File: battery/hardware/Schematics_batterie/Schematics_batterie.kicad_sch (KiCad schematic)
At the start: 45 parts, among them IC1 BQ25185DLHR, J1 USB_C_Receptacle_USB2.0_16P, J2 Conn_01x02, J3 Conn_01x02, J4 Conn_ST_STDC14, J5 Conn_01x02, U1 BU33SD5WG-TR, U2 STM32G431KBTx, U3 USBLC6-2SC6

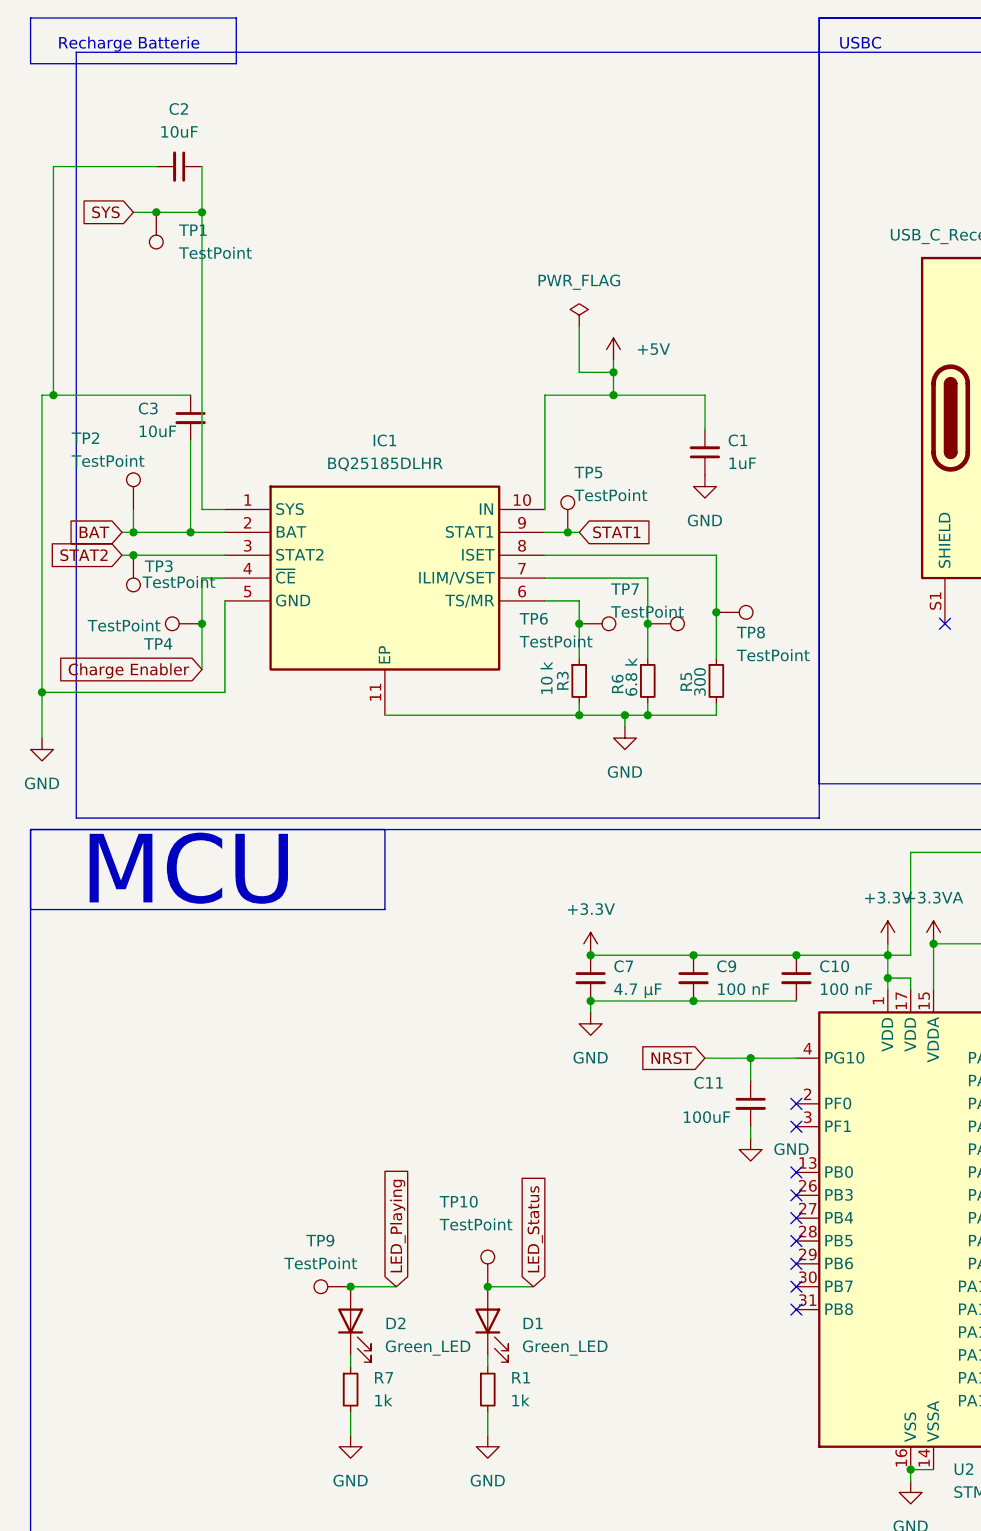
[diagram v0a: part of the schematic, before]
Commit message: derniers branchements et isolation des textes
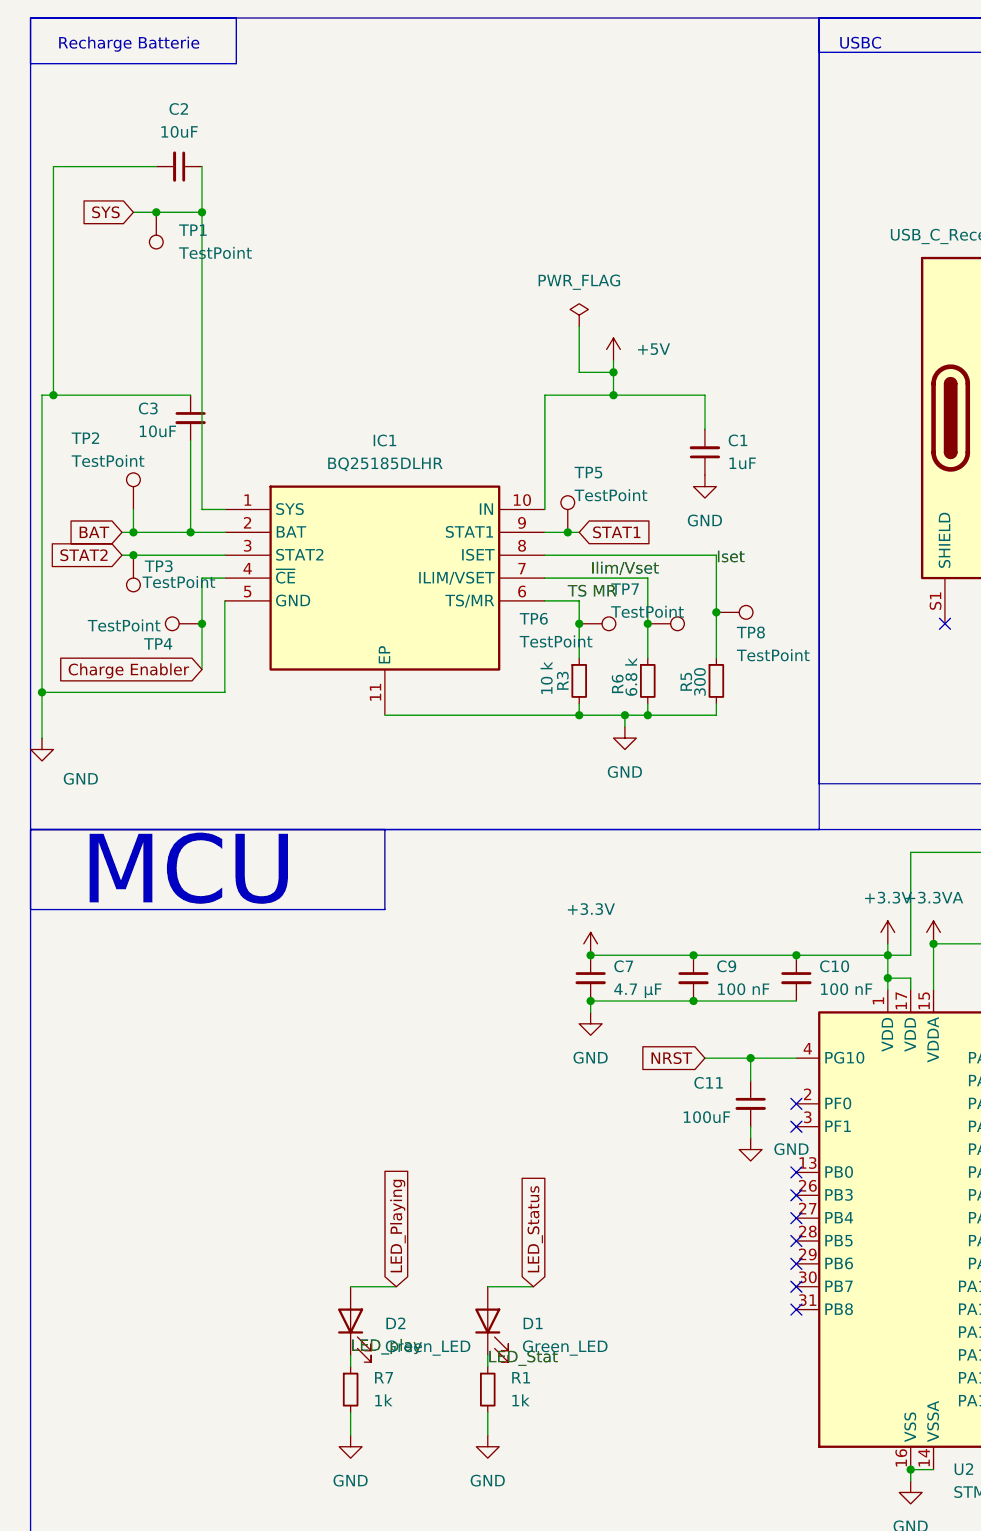
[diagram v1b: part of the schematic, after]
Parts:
- removed TP10, TP9: TestPoint, TestPoint:TestPoint_Pad_D2.0mm, symbol Connector:TestPoint
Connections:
- net TS MR: now reaches IC1.6 (TS/MR), R3.1, TP6.1
- net LED_play: now reaches D2.1 (K), R7.1
- net Ilim/Vset: now reaches IC1.7 (ILIM/VSET), R6.1, TP7.1
- net Iset: now reaches IC1.8 (ISET), R5.1, TP8.1
- net LED_Stat: now reaches D1.1 (K), R1.1
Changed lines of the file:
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@@
 	)
 	(junction
-		(at 55.88 163.83)
-		(diameter 0)
-		(color 0 0 0 0)
-	)
-	(junction
 		(at 100.33 138.43)
 		(diameter 0)
@@
 	)
 	(junction
-		(at 71.12 163.83)
-		(diameter 0)
-		(color 0 0 0 0)
-	)
-	(junction
 		(at 250.19 154.94)
 		(diameter 0)
@@
 	)
 	(rectangle
-		(start 25.4 26.67)
-		(end 107.95 111.76)
+		(start 20.32 22.86)
+		(end 107.95 113.03)
 		(stroke
 			(width 0)
@@
 		)
 	)
+	(label "Ilim{slash}Vset"
+		(at 82.55 85.09 0)
+		(effects
+			(font
+				(size 1.27 1.27)
+			)
+			(justify left bottom)
+		)
+	)
+	(label "TS MR"
+		(at 80.01 87.63 0)
+		(effects
+			(font
+				(size 1.27 1.27)
+			)
+			(justify left bottom)
+		)
+	)
+	(label "LED_Stat"
+		(at 71.12 172.72 0)
+		(effects
+			(font
+				(size 1.27 1.27)
+			)
+			(justify left bottom)
+		)
+	)
 	(label "VIN"
 		(at 187.96 133.35 0)
@@
 		)
 	)
+	(label "Iset"
+		(at 96.52 83.82 0)
+		(effects
+			(font
+				(size 1.27 1.27)
+			)
+			(justify left bottom)
+		)
+	)
+	(label "LED_play"
+		(at 55.88 171.45 0)
+		(effects
+			(font
+				(size 1.27 1.27)
+			)
+			(justify left bottom)
+		)
+	)
 	(global_label "BAT"
 		(shape input)
@@
 	)
 	(symbol
-		(lib_id "Connector:TestPoint")
-		(at 55.88 163.83 90)
-		(unit 1)
-		(exclude_from_sim no)
-		(in_bom yes)
-		(on_board yes)
-		(dnp no)
-		(fields_autoplaced yes)
-		(property "Reference" "TP9"
-			(at 52.578 158.75 90)
-			(effects
-				(font
-					(size 1.27 1.27)
-				)
-			)
-		)
-		(property "Value" "TestPoint"
-			(at 52.578 161.29 90)
-			(effects
-				(font
-					(size 1.27 1.27)
-				)
-			)
-		)
-		(property "Footprint" "TestPoint:TestPoint_Pad_D2.0mm"
-			(at 55.88 158.75 0)
-			(effects
-				(font
-					(size 1.27 1.27)
-				)
-				(hide yes)
-			)
-		)
-		(property "Datasheet" "~"
-			(at 55.88 158.75 0)
-			(effects
-				(font
-					(size 1.27 1.27)
-				)
-				(hide yes)
-			)
-		)
-		(property "Description" "test point"
-			(at 55.88 163.83 0)
-			(effects
-				(font
-					(size 1.27 1.27)
-				)
-				(hide yes)
-			)
-		)
-		(pin "1"
-		)
-		(instances
-			(project "Schematics_batterie"
-				(path "/4fbe78ef-b629-4e84-bfa0-c62113a81c93"
-					(reference "TP9")
-					(unit 1)
-				)
-			)
-		)
-	)
-	(symbol
 		(lib_id "Device:R_Small")
 		(at 152.4 59.69 270)
@@
 	)
 	(symbol
-		(lib_id "Connector:TestPoint")
-		(at 71.12 163.83 0)
-		(unit 1)
-		(exclude_from_sim no)
-		(in_bom yes)
-		(on_board yes)
-		(dnp no)
-		(property "Reference" "TP10"
-			(at 65.786 154.432 0)
-			(effects
-				(font
-					(size 1.27 1.27)
-				)
-				(justify left)
-			)
-		)
-		(property "Value" "TestPoint"
-			(at 65.786 156.972 0)
-			(effects
-				(font
-					(size 1.27 1.27)
-				)
-				(justify left)
-			)
-		)
-		(property "Footprint" "TestPoint:TestPoint_Pad_D2.0mm"
-			(at 76.2 163.83 0)
-			(effects
-				(font
-					(size 1.27 1.27)
-				)
-				(hide yes)
-			)
-		)
-		(property "Datasheet" "~"
-			(at 76.2 163.83 0)
-			(effects
-				(font
-					(size 1.27 1.27)
-				)
-				(hide yes)
-			)
-		)
-		(property "Description" "test point"
-			(at 71.12 163.83 0)
-			(effects
-				(font
-					(size 1.27 1.27)
-				)
-				(hide yes)
-			)
-		)
-		(pin "1"
-		)
-		(instances
-			(project "Schematics_batterie"
-				(path "/4fbe78ef-b629-4e84-bfa0-c62113a81c93"
-					(reference "TP10")
-					(unit 1)
-				)
-			)
-		)
-	)
-	(symbol
 		(lib_id "power:GND")
 		(at 21.59 102.87 0)
@@
 		)
 		(property "Value" "GND"
-			(at 21.59 107.95 0)
+			(at 25.908 107.442 0)
 			(effects
 				(font
